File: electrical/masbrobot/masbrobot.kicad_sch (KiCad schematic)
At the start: 50 parts, among them J1 TYPE-C-31-M-12, J2 connector battery 2S Li-Po, J3 Micro_SD_Card, J4 IO, J5 Conn_01x06, J6 Conn_01x06, J7 OLED_128x64_I2C, Q1 S8050, Q2 S8050, SW1 reset, SW2 boot, U1 CH340G, U2 MPU-6050, U3 ESP32-WROOM-32D, U4 L298P, U5 AMS1117-5.0, U6 AMS1117-3.3

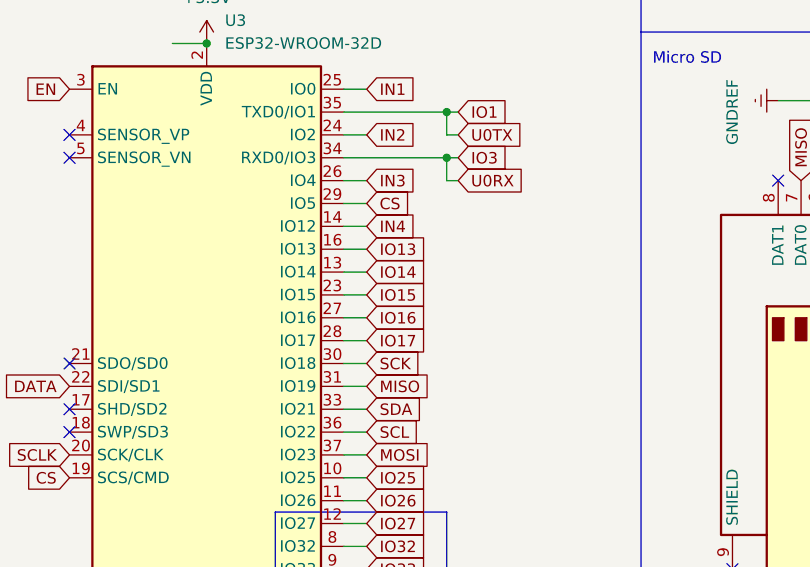
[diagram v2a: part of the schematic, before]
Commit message: update smentara
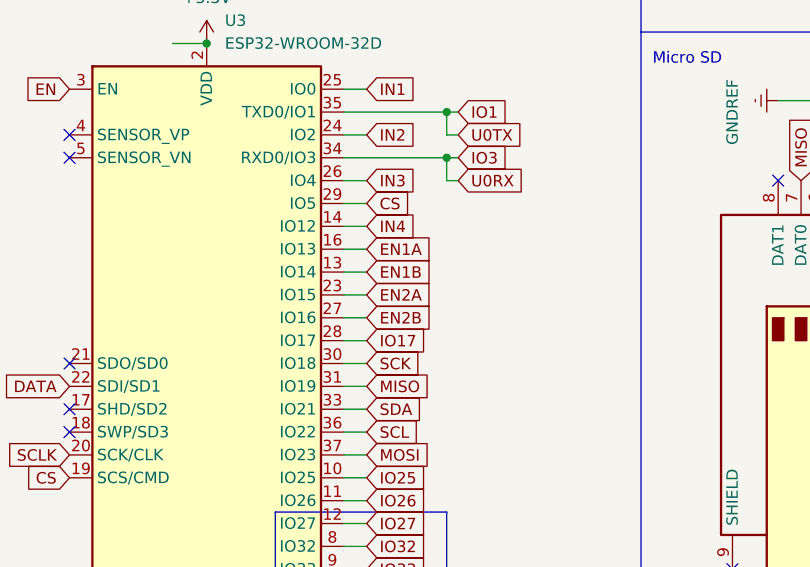
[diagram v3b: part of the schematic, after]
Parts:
- J2: footprint Connector_JST:JST_XH_S3B-XH-A-1_1x03_P2.50mm_Horizontal -> Connector_JST:JST_XH_B3B-XH-A_1x03_P2.50mm_Vertical
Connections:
- net IO13 is gone; now on net EN1A: U3.16 (IO13)
- net IO14 is gone; now on net EN1B: U3.13 (IO14)
- net IO15 is gone; now on net EN2A: U3.23 (IO15)
- net IO16 is gone; now on net EN2B: U3.27 (IO16)
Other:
- title: Schematic Masbrobot, PCB 1 -> Schematic Masbrobot
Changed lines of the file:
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@@
   (paper "User" 279.4 279.4)
   (title_block
-    (title "Schematic Masbrobot, PCB 1")
+    (title "Schematic Masbrobot")
     (date "2023-05-31")
     (rev "0.1")
@@
   )
   (wire (pts (xy 104.14 87.63) (xy 104.14 101.6))
-    (stroke (width 0) (type default))
+    (stroke (width 0) (type default) (color 255 0 7 1))
   )
   (polyline (pts (xy 182.88 167.64) (xy 182.88 77.47))
@@
   )
   (wire (pts (xy 64.77 87.63) (xy 104.14 87.63))
-    (stroke (width 0) (type default))
+    (stroke (width 0) (type default) (color 255 0 2 1))
   )
   (wire (pts (xy 149.86 138.43) (xy 152.4 138.43))
@@
     (effects (font (size 1.27 1.27)) (justify left bottom))
   )
-  (global_label "IO15" (shape input) (at 152.4 115.57 0) (fields_autoplaced)
-    (effects (font (size 1.27 1.27)) (justify left))
-    (property "Intersheetrefs" "${INTERSHEET_REFS}" (at 159.1674 115.4906 0)
+  (global_label "EN2A" (shape input) (at 152.4 115.57 0) (fields_autoplaced)
+    (effects (font (size 1.27 1.27)) (justify left))
+    (property "Intersheetrefs" "${INTERSHEET_REFS}" (at 160.0834 115.57 0)
       (effects (font (size 1.27 1.27)) (justify left) hide)
     )
@@
     )
   )
-  (global_label "IO13" (shape input) (at 152.4 110.49 0) (fields_autoplaced)
-    (effects (font (size 1.27 1.27)) (justify left))
-    (property "Intersheetrefs" "${INTERSHEET_REFS}" (at 159.1674 110.4106 0)
-      (effects (font (size 1.27 1.27)) (justify left) hide)
-    )
-  )
-  (global_label "IO16" (shape input) (at 152.4 118.11 0) (fields_autoplaced)
-    (effects (font (size 1.27 1.27)) (justify left))
-    (property "Intersheetrefs" "${INTERSHEET_REFS}" (at 159.1674 118.0306 0)
+  (global_label "EN1A" (shape input) (at 152.4 110.49 0) (fields_autoplaced)
+    (effects (font (size 1.27 1.27)) (justify left))
+    (property "Intersheetrefs" "${INTERSHEET_REFS}" (at 160.0834 110.49 0)
+      (effects (font (size 1.27 1.27)) (justify left) hide)
+    )
+  )
+  (global_label "EN2B" (shape input) (at 152.4 118.11 0) (fields_autoplaced)
+    (effects (font (size 1.27 1.27)) (justify left))
+    (property "Intersheetrefs" "${INTERSHEET_REFS}" (at 160.2648 118.11 0)
       (effects (font (size 1.27 1.27)) (justify left) hide)
     )
@@
     )
   )
-  (global_label "IO14" (shape input) (at 152.4 113.03 0) (fields_autoplaced)
-    (effects (font (size 1.27 1.27)) (justify left))
-    (property "Intersheetrefs" "${INTERSHEET_REFS}" (at 159.1674 112.9506 0)
+  (global_label "EN1B" (shape input) (at 152.4 113.03 0) (fields_autoplaced)
+    (effects (font (size 1.27 1.27)) (justify left))
+    (property "Intersheetrefs" "${INTERSHEET_REFS}" (at 160.2648 113.03 0)
       (effects (font (size 1.27 1.27)) (justify left) hide)
     )
@@
       (effects (font (size 1.27 1.27)))
     )
-    (property "Footprint" "Connector_JST:JST_XH_S3B-XH-A-1_1x03_P2.50mm_Horizontal" (at 156.21 66.04 0)
+    (property "Footprint" "Connector_JST:JST_XH_B3B-XH-A_1x03_P2.50mm_Vertical" (at 156.21 66.04 0)
       (effects (font (size 1.27 1.27)) hide)
     )
